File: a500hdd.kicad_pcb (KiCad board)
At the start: 2 copper layers, 47.6 x 111.1 mm, 29 parts, among them U1 ata_connector, U3 74LS04, U4 a500exp, U5 74LS00, U6 74LS08, U7 74LS08

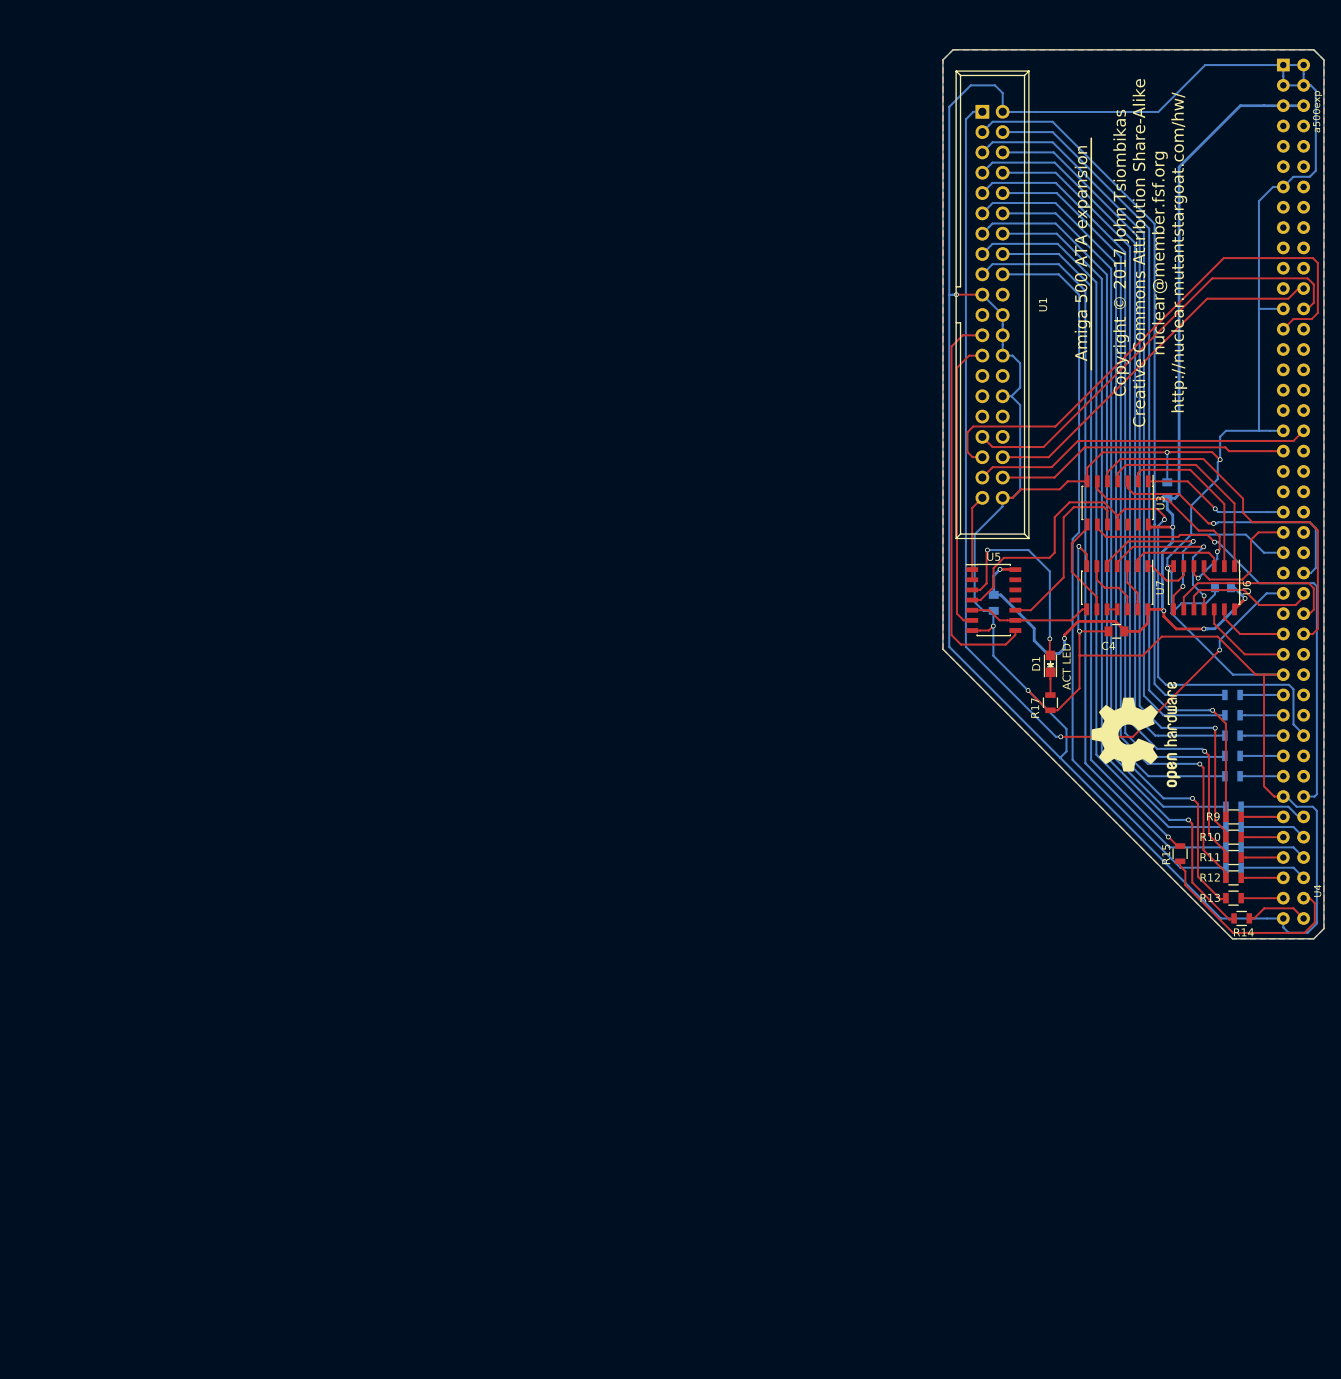
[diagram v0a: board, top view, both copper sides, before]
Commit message: Rev2 PCB, migrated do KiCad5
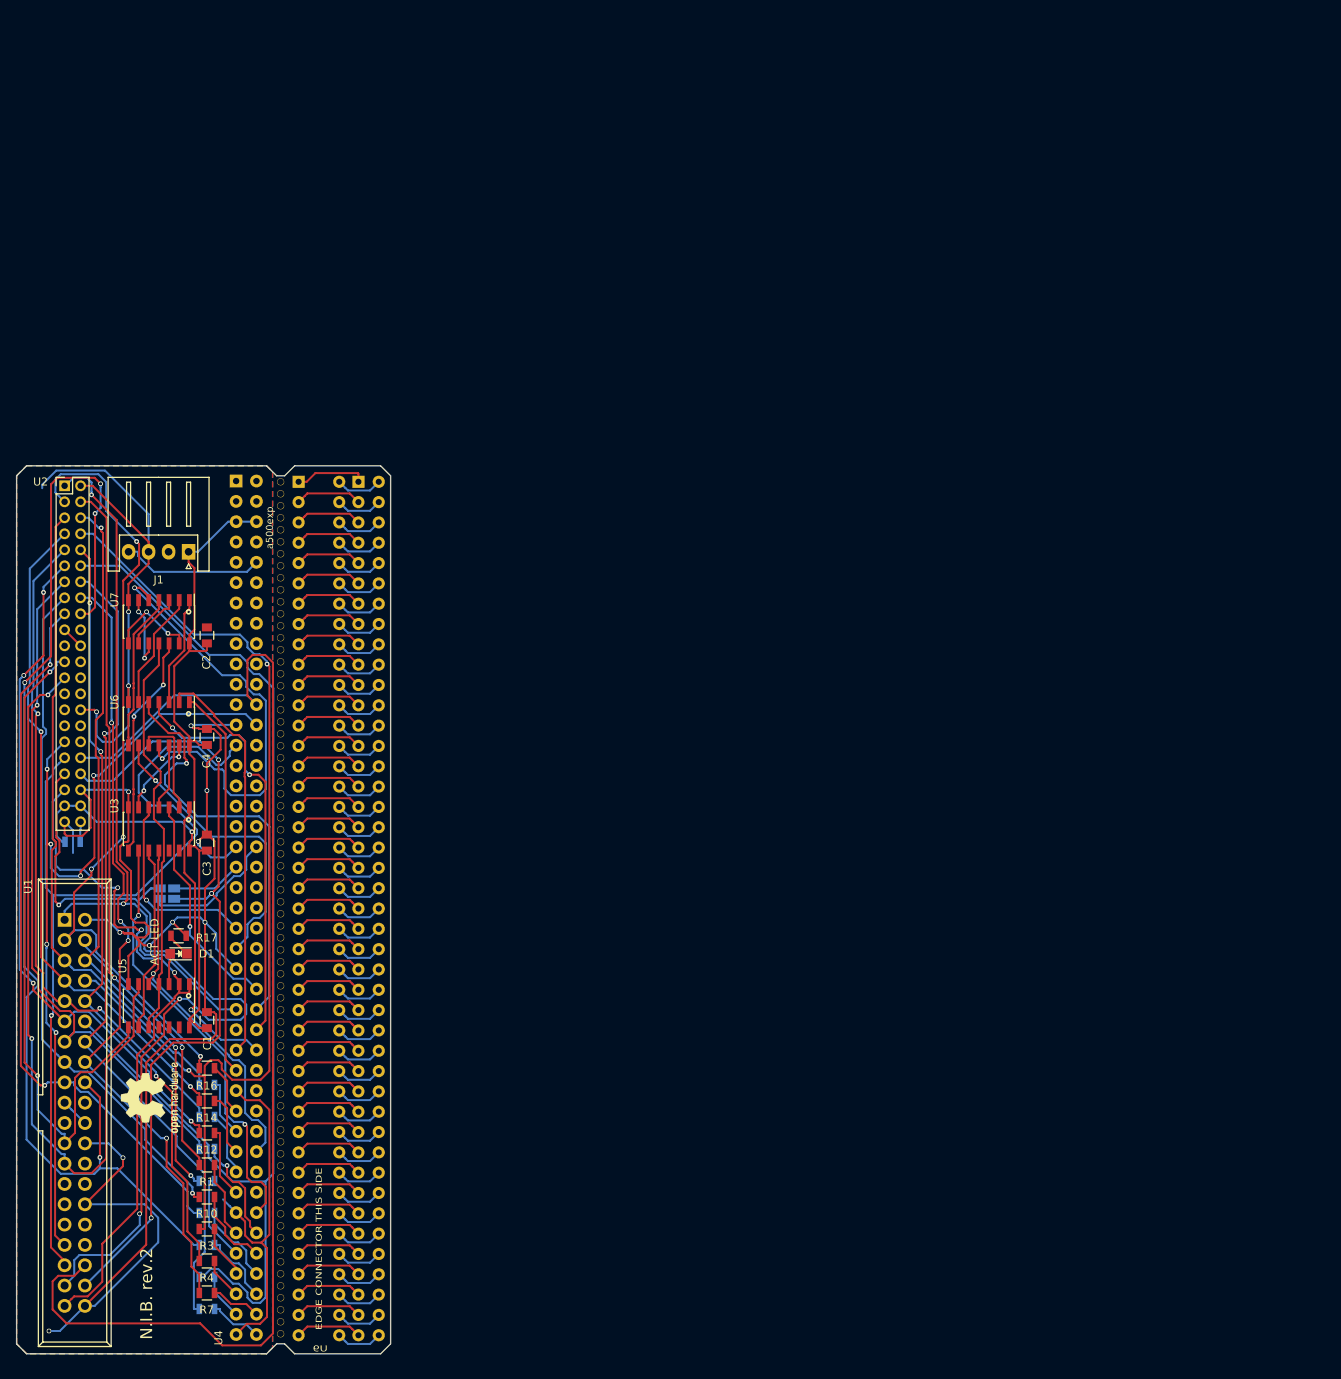
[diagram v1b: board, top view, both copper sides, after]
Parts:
- removed the REF*** at (229.2, 112.9)
- added J1: Conn_01x04_Male, Connector_JST:JST_XH_S04B-XH-A_1x04_P2.50mm_Horizontal, F.Cu at (110.8, 90.1)
- added JP1: SolderJumper_2_Bridged, Jumper:SolderJumper-2_P1.3mm_Open_Pad1.0x1.5mm, B.Cu at (107.2, 132.8)
- added JP2: SolderJumper_2_Bridged, Jumper:SolderJumper-2_P1.3mm_Open_Pad1.0x1.5mm, B.Cu at (109.0, 132.8)
- added R18: 4k7, Resistors_SMD:R_0805, B.Cu at (96.3, 126.3)
- added REF**: drill, a500hdd:drill, F.Cu at (122.3, 187.8)
- added REF**: drill, a500hdd:drill, F.Cu at (122.3, 174.3)
- added REF**: drill, a500hdd:drill, F.Cu at (122.3, 172.8)
- added REF**: drill, a500hdd:drill, F.Cu at (122.3, 169.8)
- added REF**: drill, a500hdd:drill, F.Cu at (122.3, 171.3)
- added REF**: drill, a500hdd:drill, F.Cu at (122.3, 166.8)
- added REF**: drill, a500hdd:drill, F.Cu at (122.3, 168.3)
- added REF**: drill, a500hdd:drill, F.Cu at (122.3, 163.8)
- added REF**: drill, a500hdd:drill, F.Cu at (122.3, 165.3)
- added REF**: drill, a500hdd:drill, F.Cu at (122.3, 160.8)
- added REF**: drill, a500hdd:drill, F.Cu at (122.3, 162.3)
- added REF**: drill, a500hdd:drill, F.Cu at (122.3, 186.3)
- added REF**: drill, a500hdd:drill, F.Cu at (122.3, 157.8)
- added REF**: drill, a500hdd:drill, F.Cu at (122.3, 159.3)
- added REF**: drill, a500hdd:drill, F.Cu at (122.3, 154.8)
- added REF**: drill, a500hdd:drill, F.Cu at (122.3, 156.3)
- added REF**: drill, a500hdd:drill, F.Cu at (122.3, 151.8)
- added REF**: drill, a500hdd:drill, F.Cu at (122.3, 153.3)
- added REF**: drill, a500hdd:drill, F.Cu at (122.3, 150.3)
- added REF**: drill, a500hdd:drill, F.Cu at (122.3, 148.8)
- added REF**: drill, a500hdd:drill, F.Cu at (122.3, 147.3)
- added REF**: drill, a500hdd:drill, F.Cu at (122.3, 145.8)
- added REF**: drill, a500hdd:drill, F.Cu at (122.3, 184.8)
- added REF**: drill, a500hdd:drill, F.Cu at (122.3, 144.3)
- added REF**: drill, a500hdd:drill, F.Cu at (122.3, 142.8)
- added REF**: drill, a500hdd:drill, F.Cu at (122.3, 141.3)
- added REF**: drill, a500hdd:drill, F.Cu at (122.3, 139.8)
- added REF**: drill, a500hdd:drill, F.Cu at (122.3, 136.8)
- added REF**: drill, a500hdd:drill, F.Cu at (122.3, 138.3)
- added REF**: drill, a500hdd:drill, F.Cu at (122.3, 133.8)
- added REF**: drill, a500hdd:drill, F.Cu at (122.3, 135.3)
- added REF**: drill, a500hdd:drill, F.Cu at (122.3, 130.8)
- added REF**: drill, a500hdd:drill, F.Cu at (122.3, 132.3)
- added REF**: drill, a500hdd:drill, F.Cu at (122.3, 181.8)
- added REF**: drill, a500hdd:drill, F.Cu at (122.3, 129.3)
- added REF**: drill, a500hdd:drill, F.Cu at (122.3, 127.8)
- added REF**: drill, a500hdd:drill, F.Cu at (122.3, 126.3)
- added REF**: drill, a500hdd:drill, F.Cu at (122.3, 124.8)
- added REF**: drill, a500hdd:drill, F.Cu at (122.3, 123.3)
- added REF**: drill, a500hdd:drill, F.Cu at (122.3, 121.8)
- added REF**: drill, a500hdd:drill, F.Cu at (122.3, 120.3)
- added REF**: drill, a500hdd:drill, F.Cu at (122.3, 118.8)
- added REF**: drill, a500hdd:drill, F.Cu at (122.3, 117.3)
- added REF**: drill, a500hdd:drill, F.Cu at (122.3, 115.8)
- added REF**: drill, a500hdd:drill, F.Cu at (122.3, 183.3)
- added REF**: drill, a500hdd:drill, F.Cu at (122.3, 114.3)
- added REF**: drill, a500hdd:drill, F.Cu at (122.3, 112.8)
- added REF**: drill, a500hdd:drill, F.Cu at (122.3, 111.3)
- added REF**: drill, a500hdd:drill, F.Cu at (122.3, 109.8)
- added REF**: drill, a500hdd:drill, F.Cu at (122.3, 108.3)
- added REF**: drill, a500hdd:drill, F.Cu at (122.3, 106.8)
- added REF**: drill, a500hdd:drill, F.Cu at (122.3, 105.3)
- added REF**: drill, a500hdd:drill, F.Cu at (122.3, 103.8)
- added REF**: drill, a500hdd:drill, F.Cu at (122.3, 102.3)
- added REF**: drill, a500hdd:drill, F.Cu at (122.3, 100.8)
- added REF**: drill, a500hdd:drill, F.Cu at (122.3, 178.8)
- added REF**: drill, a500hdd:drill, F.Cu at (122.3, 99.3)
- added REF**: drill, a500hdd:drill, F.Cu at (122.3, 97.8)
- added REF**: drill, a500hdd:drill, F.Cu at (122.3, 96.3)
- added REF**: drill, a500hdd:drill, F.Cu at (122.3, 94.8)
- added REF**: drill, a500hdd:drill, F.Cu at (122.3, 93.3)
- added REF**: drill, a500hdd:drill, F.Cu at (122.3, 91.8)
- added REF**: drill, a500hdd:drill, F.Cu at (122.3, 90.3)
- added REF**: drill, a500hdd:drill, F.Cu at (122.3, 88.8)
- added REF**: drill, a500hdd:drill, F.Cu at (122.3, 87.3)
- added REF**: drill, a500hdd:drill, F.Cu at (122.3, 85.8)
- added REF**: drill, a500hdd:drill, F.Cu at (122.3, 180.3)
- added REF**: drill, a500hdd:drill, F.Cu at (122.3, 84.3)
- added REF**: drill, a500hdd:drill, F.Cu at (122.3, 82.8)
- added REF**: drill, a500hdd:drill, F.Cu at (122.3, 81.3)
- added REF**: drill, a500hdd:drill, F.Cu at (122.3, 177.3)
- added REF**: drill, a500hdd:drill, F.Cu at (122.3, 175.8)
- added REF***: OSHW-Logo2_9.8x8mm_SilkScreen, Symbol:OSHW-Logo2_9.8x8mm_SilkScreen, F.Cu at (106.1, 158.3)
- added U2: ata_connector44, Pin_Headers:Pin_Header_Straight_2x22_Pitch2.00mm, F.Cu at (95.3, 81.8)
- added U8: a500exp, a500hdd:header2x43, F.Cu at (133.3, 81.3)
- added U9: a500exp, a500hdd:A500_Expansion_slot, F.Cu at (124.6, 81.3)
- C1, C2, C3, R1, R16, R3, R4, R7: moved to F.Cu
- R11, R13, R15, R9: moved to B.Cu
- moved U1 152.8 mm to (95.3, 136.1)
- moved R7 147.1 mm to (113.1, 182.7), turned to 0 degrees
- moved R6 146.9 mm to (113.1, 184.7), turned to 0 degrees
- moved R8 145.5 mm to (113.1, 176.7), turned to 0 degrees
- moved R5 143.8 mm to (113.1, 180.7), turned to 0 degrees
- moved R4 141.8 mm to (113.1, 178.7), turned to 0 degrees
- moved U4 140.9 mm to (119.3, 134.6)
- moved R3 138.8 mm to (113.1, 174.7), turned to 0 degrees
- moved R9 137.5 mm to (113.1, 172.7), turned to 0 degrees
- moved C1 137.1 mm to (113.1, 148.6)
- moved R10 136.0 mm to (113.1, 170.7), turned to 0 degrees
- moved R2 135.7 mm to (113.1, 168.7), turned to 0 degrees
- moved R1 134.3 mm to (113.1, 166.7), turned to 0 degrees
- moved R11 133.4 mm to (113.1, 164.7), turned to 0 degrees
- moved R12 132.2 mm to (113.1, 162.7), turned to 0 degrees
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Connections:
- net /A18 renamed A18
- net /ACTLED renamed Net-(D1-Pad2)
- net /ATA_A0 renamed ATA_A0
- net /ATA_A1 renamed ATA_A1
- net /ATA_A2 renamed ATA_A2
- net /~ACTLED renamed ~ATA_ACTILED
- net /~AS renamed ~AS
- net /~ATA_RD renamed ~ATA_RD
- net /~ATA_WR renamed ~ATA_WR
- net /~RESET renamed ~ATA_RESET
- R1 pad 1: /D8 -> /D0
- R1 pad 2: /ATA_D0 -> Net-(R1-Pad2)
- R10 pad 1: /D1 -> /D9
- R10 pad 2: /ATA_D9 -> Net-(R10-Pad2)
- R11 pad 1: /D2 -> /D10
- R11 pad 2: /ATA_D10 -> Net-(R11-Pad2)
- R12 pad 1: /D3 -> /D11
- R12 pad 2: /ATA_D11 -> Net-(R12-Pad2)
- R13 pad 1: /D4 -> /D12
- R13 pad 2: /ATA_D12 -> Net-(R13-Pad2)
- R14 pad 1: /D5 -> /D13
- R14 pad 2: /ATA_D13 -> Net-(R14-Pad2)
- R15 pad 1: /D6 -> /D14
- R15 pad 2: /ATA_D14 -> Net-(R15-Pad2)
- R16 pad 1: /D7 -> /D15
- R16 pad 2: /ATA_D15 -> Net-(R16-Pad2)
- R2 pad 1: /D9 -> /D1
- R2 pad 2: /ATA_D1 -> Net-(R2-Pad2)
- R3 pad 1: /D10 -> /D2
- R3 pad 2: /ATA_D2 -> Net-(R3-Pad2)
- R4 pad 1: /D11 -> /D3
- R4 pad 2: /ATA_D3 -> Net-(R4-Pad2)
- R5 pad 1: /D12 -> /D4
- R5 pad 2: /ATA_D4 -> Net-(R5-Pad2)
- R6 pad 1: /D13 -> /D5
- R6 pad 2: /ATA_D5 -> Net-(R6-Pad2)
- R7 pad 1: /D14 -> /D6
- R7 pad 2: /ATA_D6 -> Net-(R7-Pad2)
- R8 pad 1: /D15 -> /D7
- R8 pad 2: /ATA_D7 -> Net-(R8-Pad2)
- R9 pad 1: /D0 -> /D8
- R9 pad 2: /ATA_D8 -> Net-(R9-Pad2)
- U1 pad 10: /ATA_D11 -> /D3
- U1 pad 11: /ATA_D3 -> /D11
- U1 pad 12: /ATA_D12 -> /D4
- U1 pad 13: /ATA_D2 -> /D10
- U1 pad 14: /ATA_D13 -> /D5
- U1 pad 15: /ATA_D1 -> /D9
- U1 pad 16: /ATA_D14 -> /D6
- U1 pad 17: /ATA_D0 -> /D8
- U1 pad 18: /ATA_D15 -> /D7
- U1 pad 20: (no net) -> Net-(U1-Pad20)
- U1 pad 21: (no net) -> Net-(U1-Pad21)
- U1 pad 27: (no net) -> Net-(U1-Pad27)
- U1 pad 28: (no net) -> Net-(U1-Pad28)
- U1 pad 29: (no net) -> Net-(U1-Pad29)
- U1 pad 3: /ATA_D7 -> /D15
- U1 pad 31: (no net) -> Net-(U1-Pad31)
- U1 pad 32: (no net) -> Net-(U1-Pad32)
- U1 pad 34: (no net) -> Net-(U1-Pad34)
- U1 pad 37: /~ATA_CS0 -> ~ATA_CS0
- U1 pad 38: /~ATA_CS1 -> ~ATA_CS1
- U1 pad 4: /ATA_D8 -> /D0
- U1 pad 5: /ATA_D6 -> /D14
- U1 pad 6: /ATA_D9 -> /D1
- U1 pad 7: /ATA_D5 -> /D13
- U1 pad 8: /ATA_D10 -> /D2
- U1 pad 9: /ATA_D4 -> /D12
- U3 pad 1: /A16 -> A21
- U3 pad 11: /R/~W -> R/~W
- U3 pad 5: /A21 -> A16
- U3 pad 8: /AS -> Net-(U3-Pad8)
- U4 pad 10: (no net) -> +12V
- U4 pad 11: (no net) -> Net-(U4-Pad11)
- U4 pad 12: (no net) -> Net-(U4-Pad12)
- U4 pad 14: (no net) -> Net-(U4-Pad14)
- U4 pad 15: (no net) -> Net-(U4-Pad15)
- U4 pad 16: (no net) -> Net-(U4-Pad16)
- U4 pad 17: (no net) -> Net-(U4-Pad17)
- U4 pad 18: (no net) -> Net-(U4-Pad18)
- U4 pad 19: (no net) -> Net-(U4-Pad19)
- U4 pad 20: (no net) -> Net-(U4-Pad20)
- U4 pad 21: (no net) -> Net-(U4-Pad21)
- U4 pad 22: (no net) -> Net-(U4-Pad22)
- U4 pad 23: (no net) -> Net-(U4-Pad23)
- U4 pad 28: (no net) -> Net-(U4-Pad28)
- U4 pad 29: (no net) -> Net-(U4-Pad29)
- U4 pad 30: (no net) -> Net-(U4-Pad30)
- U4 pad 31: (no net) -> Net-(U4-Pad31)
- U4 pad 32: (no net) -> Net-(U4-Pad32)
- U4 pad 33: (no net) -> Net-(U4-Pad33)
- U4 pad 34: (no net) -> Net-(U4-Pad34)
- U4 pad 35: (no net) -> Net-(U4-Pad35)
- U4 pad 36: (no net) -> Net-(U4-Pad36)
- U4 pad 38: /~ATA_CS0 -> ~ATA_CSA
- U4 pad 39: /~ATA_CS1 -> ~ATA_CSB
- U4 pad 40: (no net) -> Net-(U4-Pad40)
- U4 pad 41: (no net) -> Net-(U4-Pad41)
- U4 pad 42: (no net) -> Net-(U4-Pad42)
- U4 pad 43: (no net) -> Net-(U4-Pad43)
- U4 pad 44: (no net) -> Net-(U4-Pad44)
- U4 pad 45: /A16 -> A16
- U4 pad 46: (no net) -> Net-(U4-Pad46)
- U4 pad 47: /A17 -> A17
- U4 pad 48: (no net) -> Net-(U4-Pad48)
- U4 pad 50: (no net) -> Net-(U4-Pad50)
- U4 pad 51: (no net) -> Net-(U4-Pad51)
- U4 pad 54: /A19 -> A19
- U4 pad 55: (no net) -> Net-(U4-Pad55)
- U4 pad 56: /A20 -> A20
- U4 pad 57: /A22 -> A22
- U4 pad 58: /A21 -> A21
- U4 pad 59: /A23 -> A23
- U4 pad 60: (no net) -> Net-(U4-Pad60)
- U4 pad 62: (no net) -> Net-(U4-Pad62)
- U4 pad 63: /D15 -> Net-(R16-Pad2)
- U4 pad 64: (no net) -> Net-(U4-Pad64)
- U4 pad 65: /D14 -> Net-(R15-Pad2)
- U4 pad 66: (no net) -> Net-(U4-Pad66)
- U4 pad 67: /D13 -> Net-(R14-Pad2)
- U4 pad 68: /R/~W -> R/~W
- U4 pad 69: /D12 -> Net-(R13-Pad2)
- U4 pad 7: (no net) -> Net-(U4-Pad7)
- U4 pad 70: (no net) -> Net-(U4-Pad70)
- U4 pad 71: /D11 -> Net-(R12-Pad2)
- U4 pad 72: (no net) -> Net-(U4-Pad72)
- U4 pad 75: /D0 -> Net-(R1-Pad2)
- U4 pad 76: /D10 -> Net-(R11-Pad2)
- U4 pad 77: /D1 -> Net-(R2-Pad2)
- U4 pad 78: /D9 -> Net-(R10-Pad2)
- U4 pad 79: /D2 -> Net-(R3-Pad2)
- U4 pad 8: (no net) -> Net-(U4-Pad8)
- U4 pad 80: /D8 -> Net-(R9-Pad2)
- U4 pad 81: /D3 -> Net-(R4-Pad2)
- U4 pad 82: /D7 -> Net-(R8-Pad2)
- U4 pad 83: /D4 -> Net-(R5-Pad2)
- U4 pad 84: /D6 -> Net-(R7-Pad2)
- U4 pad 86: /D5 -> Net-(R6-Pad2)
- U4 pad 9: (no net) -> Net-(U4-Pad9)
- U5 pad 10: Net-(U3-Pad10) -> ENABLE
- U5 pad 4: /R/~W -> ENABLE
- U5 pad 5: /ADDREN -> R/~W
- U5 pad 9: /ADDREN -> Net-(U3-Pad10)
- U6 pad 1: Net-(U3-Pad4) -> A23
- U6 pad 10: /A19 -> Net-(U3-Pad2)
- U6 pad 12: /A23 -> Net-(U3-Pad4)
- U6 pad 13: /A22 -> Net-(U3-Pad6)
- U6 pad 2: Net-(U3-Pad2) -> A22
- U6 pad 4: /A17 -> A20
- U6 pad 5: Net-(U3-Pad6) -> A19
- U6 pad 9: /A20 -> A17
- U7 pad 1: Net-(U6-Pad6) -> Net-(U6-Pad3)
- U7 pad 11: Net-(U7-Pad10) -> ENABLE
- U7 pad 12: Net-(U7-Pad12) -> Net-(U3-Pad8)
- U7 pad 2: Net-(U6-Pad3) -> Net-(U6-Pad6)
- U7 pad 3: Net-(U7-Pad13) -> Net-(U7-Pad3)
- U7 pad 4: Net-(U6-Pad11) -> Net-(U6-Pad8)
- U7 pad 5: Net-(U6-Pad8) -> Net-(U6-Pad11)
- U7 pad 6: Net-(U7-Pad12) -> Net-(U7-Pad10)
- U7 pad 8: /ADDREN -> Net-(U7-Pad13)
- U7 pad 9: /AS -> Net-(U7-Pad3)
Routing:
- net GND: track 521.8 -> 345.2 mm, vias 8 -> 13
- net /D4: track 5.29 -> 150.5 mm
- net /D7: track 9.31 -> 148.5 mm, vias 0 -> 4
- net /D2: track 5.29 -> 132.9 mm, vias 0 -> 2
- net ATA_A2: track 46.6 -> 157.8 mm
- net ~ATA_CS0: track 0.00 -> 108.6 mm, vias 0 -> 3
- net /ATA_D11: track 104.9 -> 0.00 mm, vias 1 -> 0
- net /ATA_D9: track 104.8 -> 0.00 mm, vias 1 -> 0
- net /ATA_D10: track 104.3 -> 0.00 mm, vias 1 -> 0
- net /ATA_D8: track 104.0 -> 0.00 mm, vias 1 -> 0
- net /ATA_D12: track 103.7 -> 0.00 mm, vias 1 -> 0
- net /ATA_D13: track 103.4 -> 0.00 mm, vias 1 -> 0
- net ~ATA_CS1: track 0.00 -> 102.0 mm, vias 0 -> 3
- net /ATA_D2: track 96.0 -> 0.00 mm
- net /ATA_D4: track 95.8 -> 0.00 mm
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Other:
- board size 47.6 x 111.1 mm -> 46.8 x 111 mm
- board text added: "Amiga 500 ATA expansion - http://AmigaPorts.github.com/a500hdd/ - Copyright © 2018 AmigaPorts (amiga@eevul.net)"
- board text added: "Bassically - part of a500hdd rev.2. (http://AmigaPorts.github.com/a500hdd/)"
- board text added: "Creative Commons Attribution Share-Alike - based on work of John Tsiombikas (nuclear@member.fsf.org)"
- board text added: "Default: = ~CS~ swap: ||"
- board text added: "N.I.B. rev.2"
- board text removed: "Amiga 500 ATA expansion Copyright © 2017 John Tsiombikas Creative Commons Attribution Share-Alike nuclear@member.fsf.org http://nuclear.mutantstargoat.com/hw/"
